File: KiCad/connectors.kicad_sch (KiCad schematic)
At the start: 0 parts

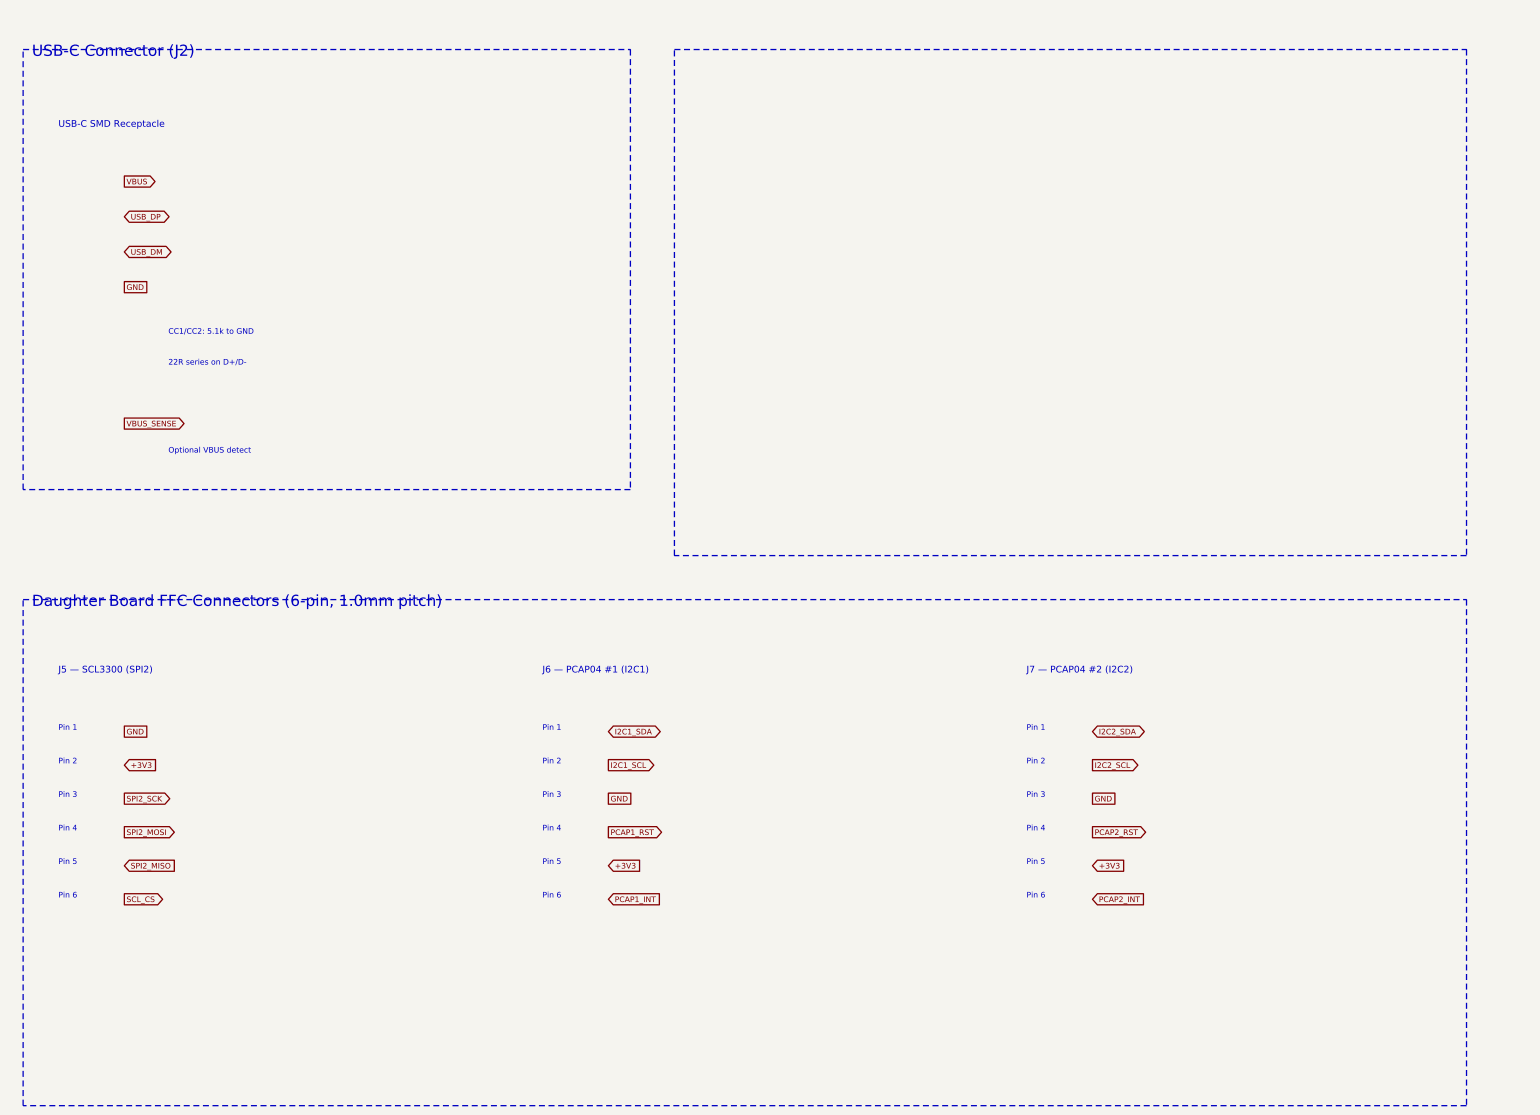
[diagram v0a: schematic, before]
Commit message: Schematic finalized
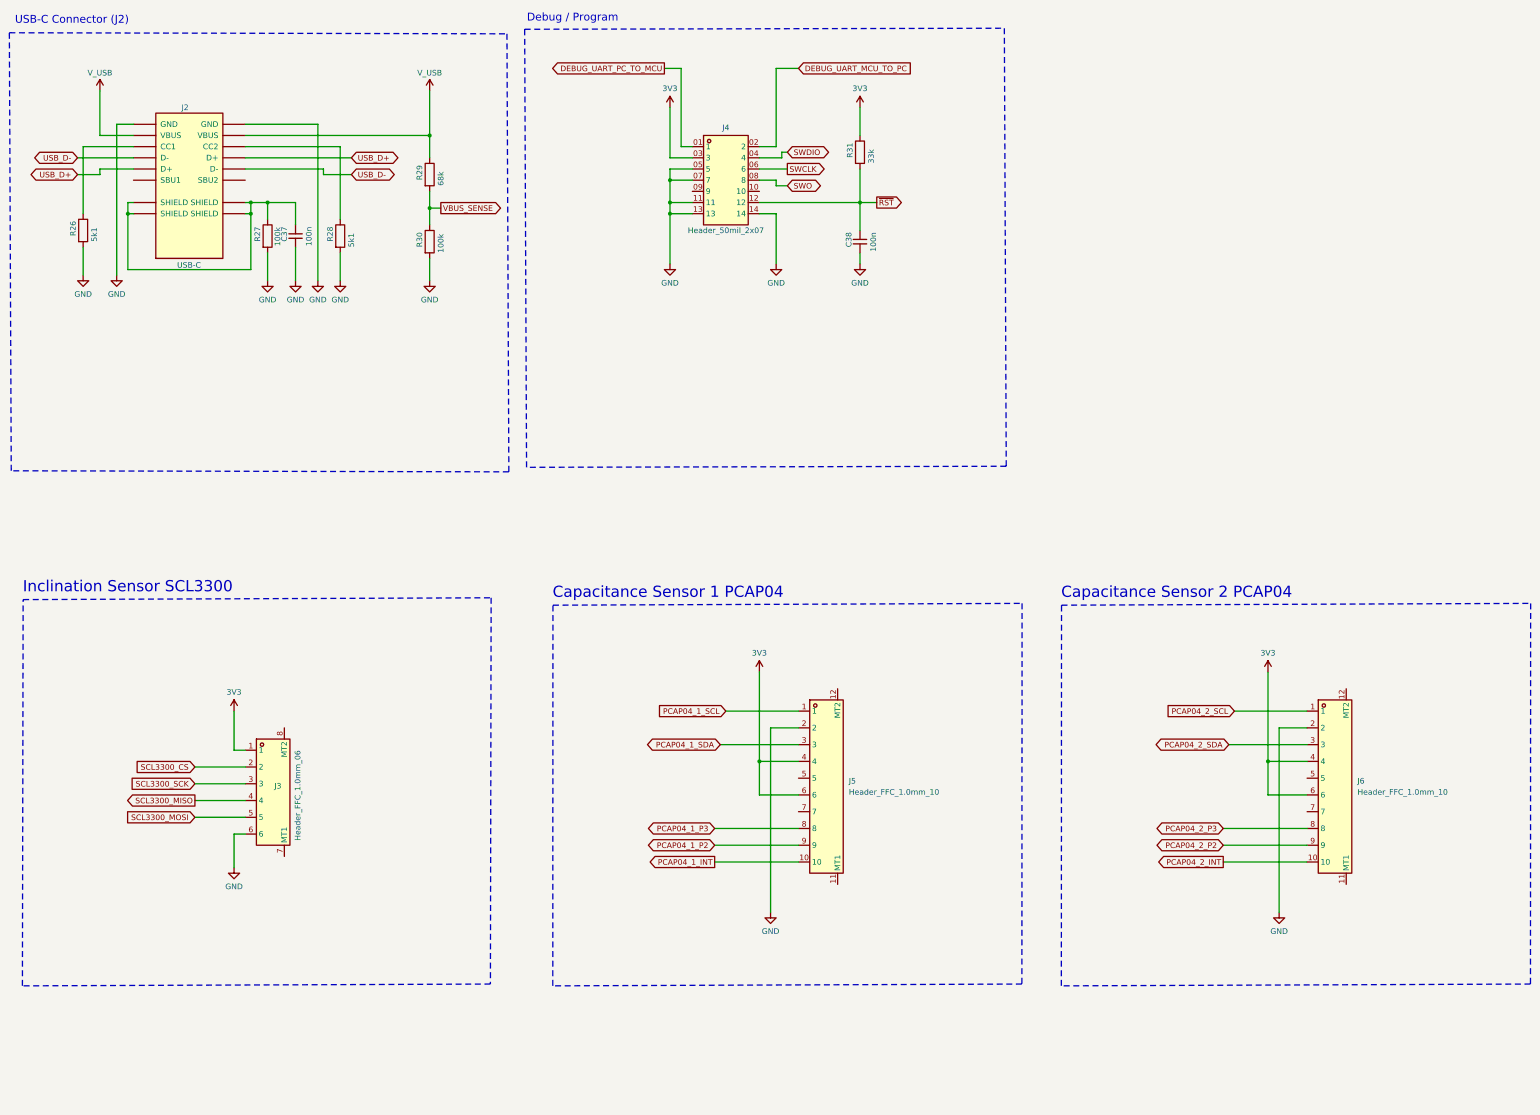
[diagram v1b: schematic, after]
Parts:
- added C37, C38: 100n, sldrnrd:C_0603, symbol sldrnrd:Capacitor/C_0603
- added J2: USB-C, sldrnrd:USB_C, symbol sldrnrd:Connector/USB/USB_C
- added J3: Header_FFC_1.0mm_06, sldrnrd:Header_FFC_1.0mm_06, symbol sldrnrd:Connector/FFC/Header_FFC_1.0mm_06
- added J4: Header_50mil_2x07, sldrnrd:Header_50mil_2x07, symbol sldrnrd:Connector/50Mil/Header_50mil_2x07
- added J5, J6: Header_FFC_1.0mm_10, sldrnrd:Header_FFC_1.0mm_10, symbol sldrnrd:Connector/FFC/Header_FFC_1.0mm_10
- added R26, R28: 5k1, sldrnrd:R_0603, symbol sldrnrd:Resistor/R_0603
- added R27, R30: 100k, sldrnrd:R_0603, symbol sldrnrd:Resistor/R_0603
- added R29: 68k, sldrnrd:R_0603, symbol sldrnrd:Resistor/R_0603
- added R31: 33k, sldrnrd:R_0603, symbol sldrnrd:Resistor/R_0603
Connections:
- net GND: now also C37.2, C38.2, J2.A1B12 (GND), J2.B1A12 (GND), J3.6, J4.05 (5), J4.07 (7), J4.11, J4.13, J4.14, J5.2, J6.2, R26.2, R27.2, R28.2, R30.2
- net VBUS_SENSE: now also R29.2, R30.1
- new net: C37.1, J2.1 (SHIELD), J2.2 (SHIELD), J2.3 (SHIELD), J2.4 (SHIELD), R27.1
- new net: J2.A5 (CC1), R26.1
- new net: J2.B5 (CC2), R28.1
- new net 3V3: J3.1, J4.03 (3), J5.4, J5.6, J6.4, J6.6, R31.1
- new net DEBUG_UART_MCU_TO_PC: J4.02 (2)
- new net DEBUG_UART_PC_TO_MCU: J4.01 (1)
- new net PCAP04_1_INT: J5.10
- new net PCAP04_1_P2: J5.9
- new net PCAP04_1_P3: J5.8
- new net PCAP04_1_SCL: J5.1
- new net PCAP04_1_SDA: J5.3
- new net PCAP04_2_INT: J6.10
- new net PCAP04_2_P2: J6.9
- new net PCAP04_2_P3: J6.8
- new net PCAP04_2_SCL: J6.1
- new net PCAP04_2_SDA: J6.3
- new net SCL3300_CS: J3.2
- new net SCL3300_MISO: J3.4
- new net SCL3300_MOSI: J3.5
- new net SCL3300_SCK: J3.3
- new net SWCLK: J4.06 (6)
- new net SWDIO: J4.04 (4)
- new net SWO: J4.08 (8)
- new net USB_D+: J2.A7 (D+), J2.B6 (D+)
- new net USB_D-: J2.A6 (D-), J2.B7 (D-)
- new net V_USB: J2.A4B9 (VBUS), J2.B4A9 (VBUS), R29.1
- new net ~{RST}: C38.1, J4.12, R31.2
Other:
- note added: "Capacitance Sensor 1 PCAP04"
- note added: "Capacitance Sensor 2 PCAP04"
- note added: "Debug / Program"
- note added: "Inclination Sensor SCL3300"
- note removed: "22R series on D+/D-"
- note removed: "CC1/CC2: 5.1k to GND"
- note removed: "Daughter Board FFC Connectors (6-pin, 1.0mm pitch)"
- note removed: "J5 — SCL3300 (SPI2)"
- note removed: "J6 — PCAP04 #1 (I2C1)"
- note removed: "J7 — PCAP04 #2 (I2C2)"
- note removed: "Optional VBUS detect"
- note removed: "Pin 1"
- note removed: "Pin 2"
- note removed: "Pin 3"
- note removed: "Pin 4"
- note removed: "Pin 5"
- note removed: "Pin 6"
- note removed: "USB-C SMD Receptacle"
